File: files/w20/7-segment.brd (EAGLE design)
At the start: 37.5 x 64.8 mm, 18 parts

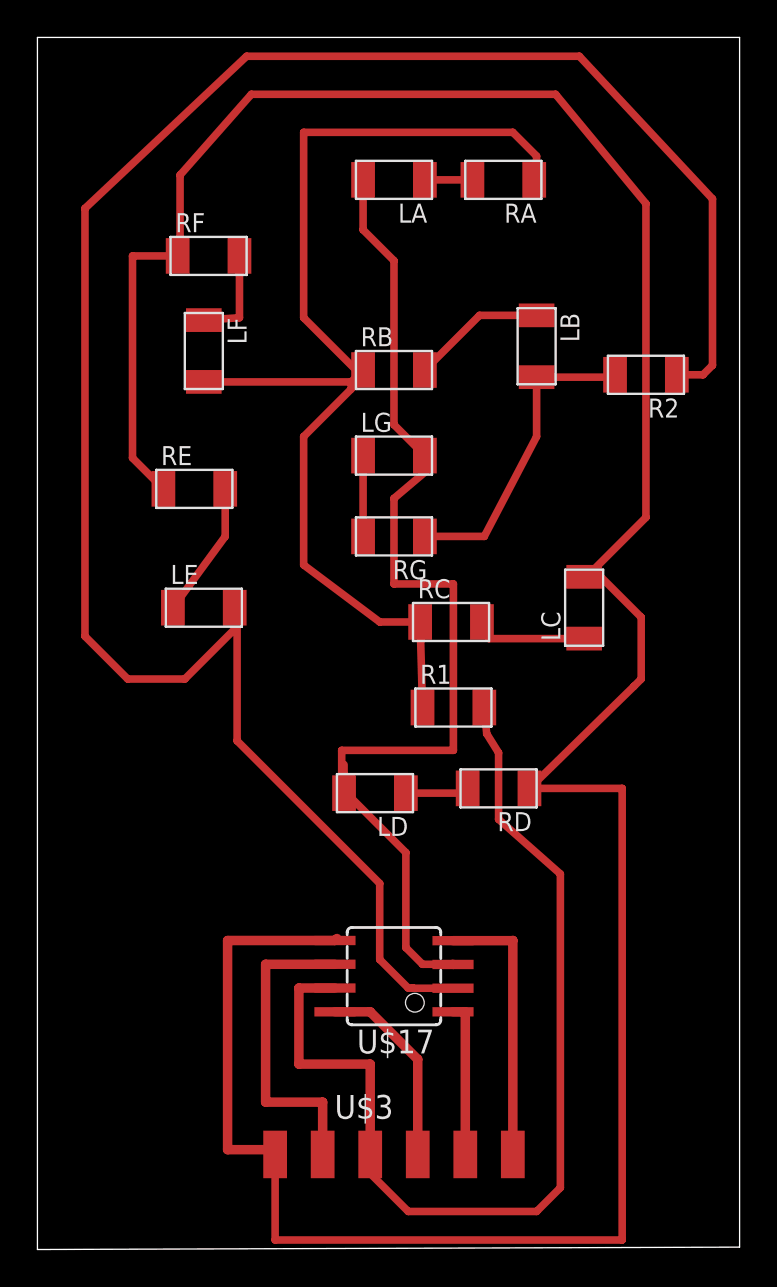
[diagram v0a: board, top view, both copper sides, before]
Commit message: vias done
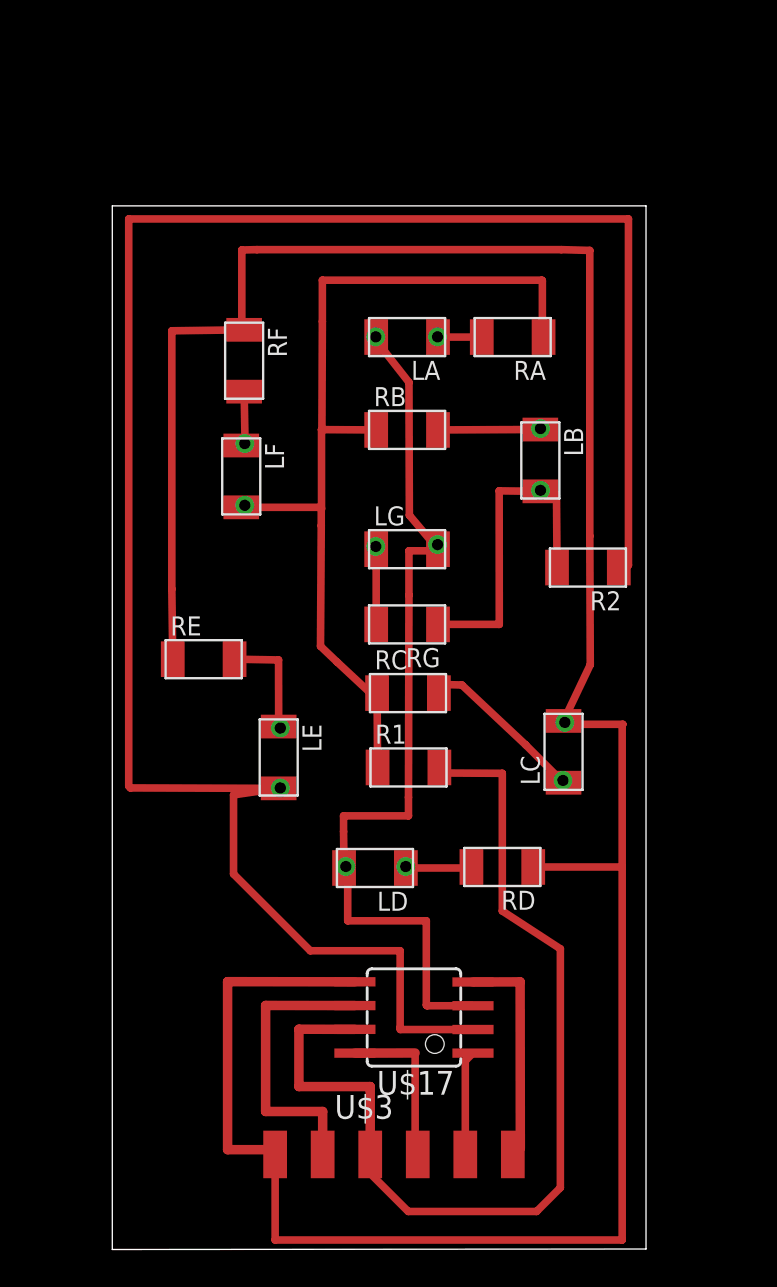
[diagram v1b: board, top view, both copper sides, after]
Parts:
- moved R2 10.8 mm to (27.6, 35.7)
- moved RE 9.11 mm to (7.10, 30.8)
- moved LE 8.94 mm to (11.1, 25.5), turned to 270 degrees
- moved LA 8.43 mm to (18.0, 48.0)
- moved RA 8.41 mm to (23.6, 48.0)
- moved LC 7.78 mm to (26.3, 25.8)
- moved LF 6.99 mm to (9.11, 40.5)
- moved LB 6.10 mm to (25.1, 41.4)
- moved RF 5.91 mm to (9.27, 46.7), turned to 270 degrees
- moved LG 5.05 mm to (18.0, 36.7)
- moved RG 4.75 mm to (18.0, 32.6)
- moved RC 4.44 mm to (18.0, 29.0)
- moved RD 4.20 mm to (23.1, 19.7)
- moved LD 4.00 mm to (16.3, 19.6)
- moved R1 4.00 mm to (18.0, 25.0)
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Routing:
- net MOSI: track 158.4 -> 147.1 mm
- net SCK: track 113.1 -> 102.1 mm
- net PB4: track 57.2 -> 48.7 mm
- net N$3: track 6.05 -> 9.23 mm
- net GND: track 14.6 -> 11.9 mm
- net RST: track 8.28 -> 5.58 mm
- net N$6: track 5.21 -> 3.06 mm
- net VCC: track 10.6 -> 8.70 mm
- net N$2: track 7.18 -> 5.47 mm
- net N$5: track 7.26 -> 5.91 mm
- net MISO: track 16.9 -> 15.8 mm
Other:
- board size 37.5 x 64.8 mm -> 28.5 x 55.8 mm
